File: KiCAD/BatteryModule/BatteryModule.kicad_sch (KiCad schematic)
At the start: 11 parts, among them J2 DF1B-2S-2.5R, J3 DF11-8DP-2DS

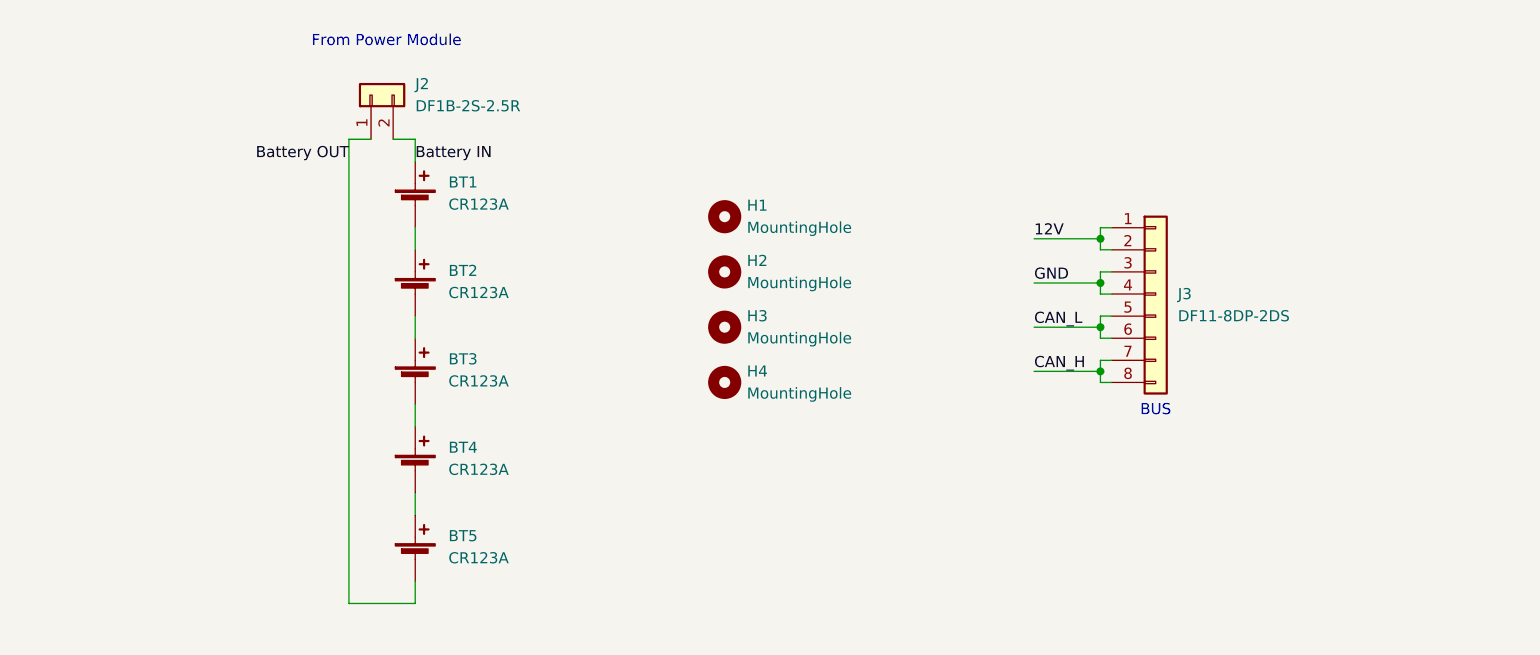
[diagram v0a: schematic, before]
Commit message: 3Dモデルを組み合わせて結合試験する．
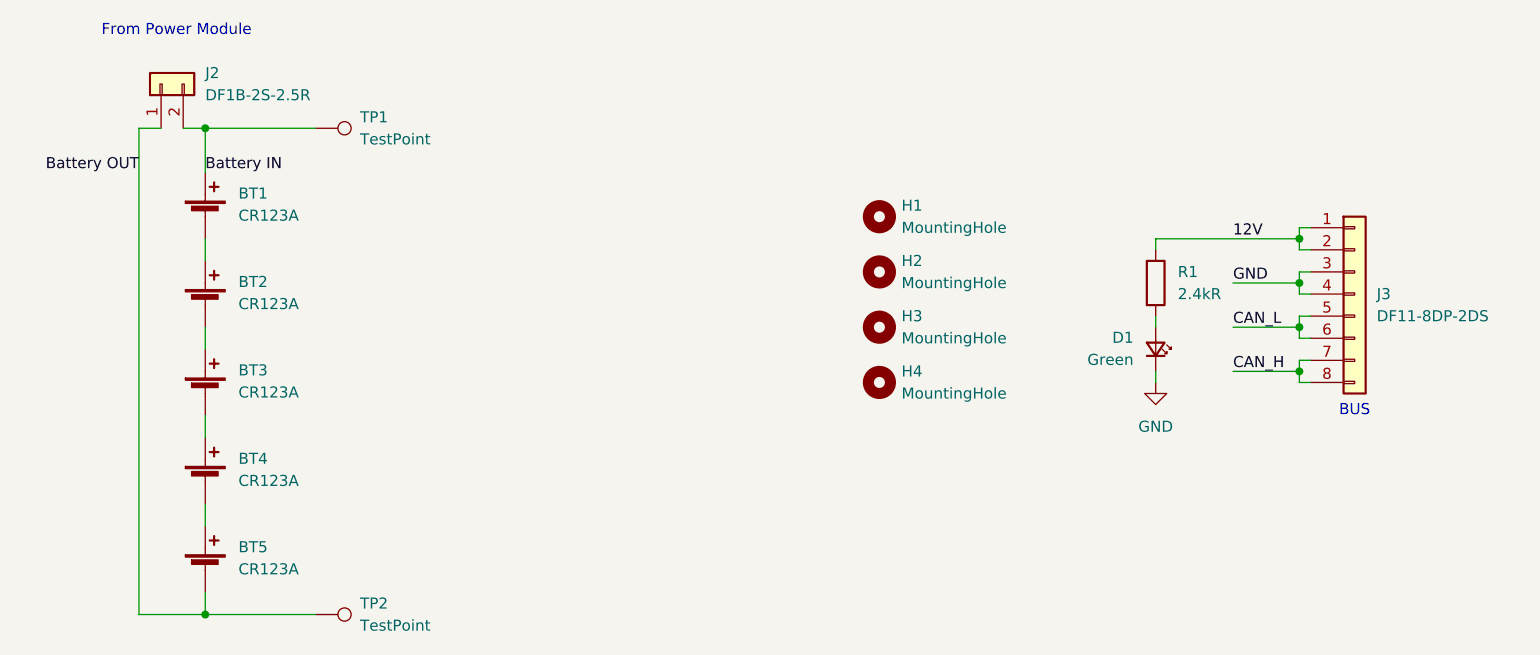
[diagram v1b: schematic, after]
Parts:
- added D1: Green, LED_SMD:LED_0603_1608Metric_Pad1.05x0.95mm_HandSolder, symbol Device:LED_Small
- added R1: 2.4kR, Resistor_SMD:R_0603_1608Metric_Pad0.98x0.95mm_HandSolder, symbol Device:R
- added TP1, TP2: TestPoint, TestPoint:TestPoint_THTPad_D2.0mm_Drill1.0mm, symbol Connector:TestPoint
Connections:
- net 12V: now also R1.1
- net Battery IN: now also TP1.1
- net Battery OUT: now also TP2.1
- net GND: now also D1.1 (K)
- new net: D1.2 (A), R1.2
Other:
- moved on the sheet: BT1, BT2, BT3, BT4, BT5, H1, H2, H3, H4, J2, J3
